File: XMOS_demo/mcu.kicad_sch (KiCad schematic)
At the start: 30 parts, among them J1 XSYS2 DEBUG CONNECTOR, U1 U316-1024-QF60B

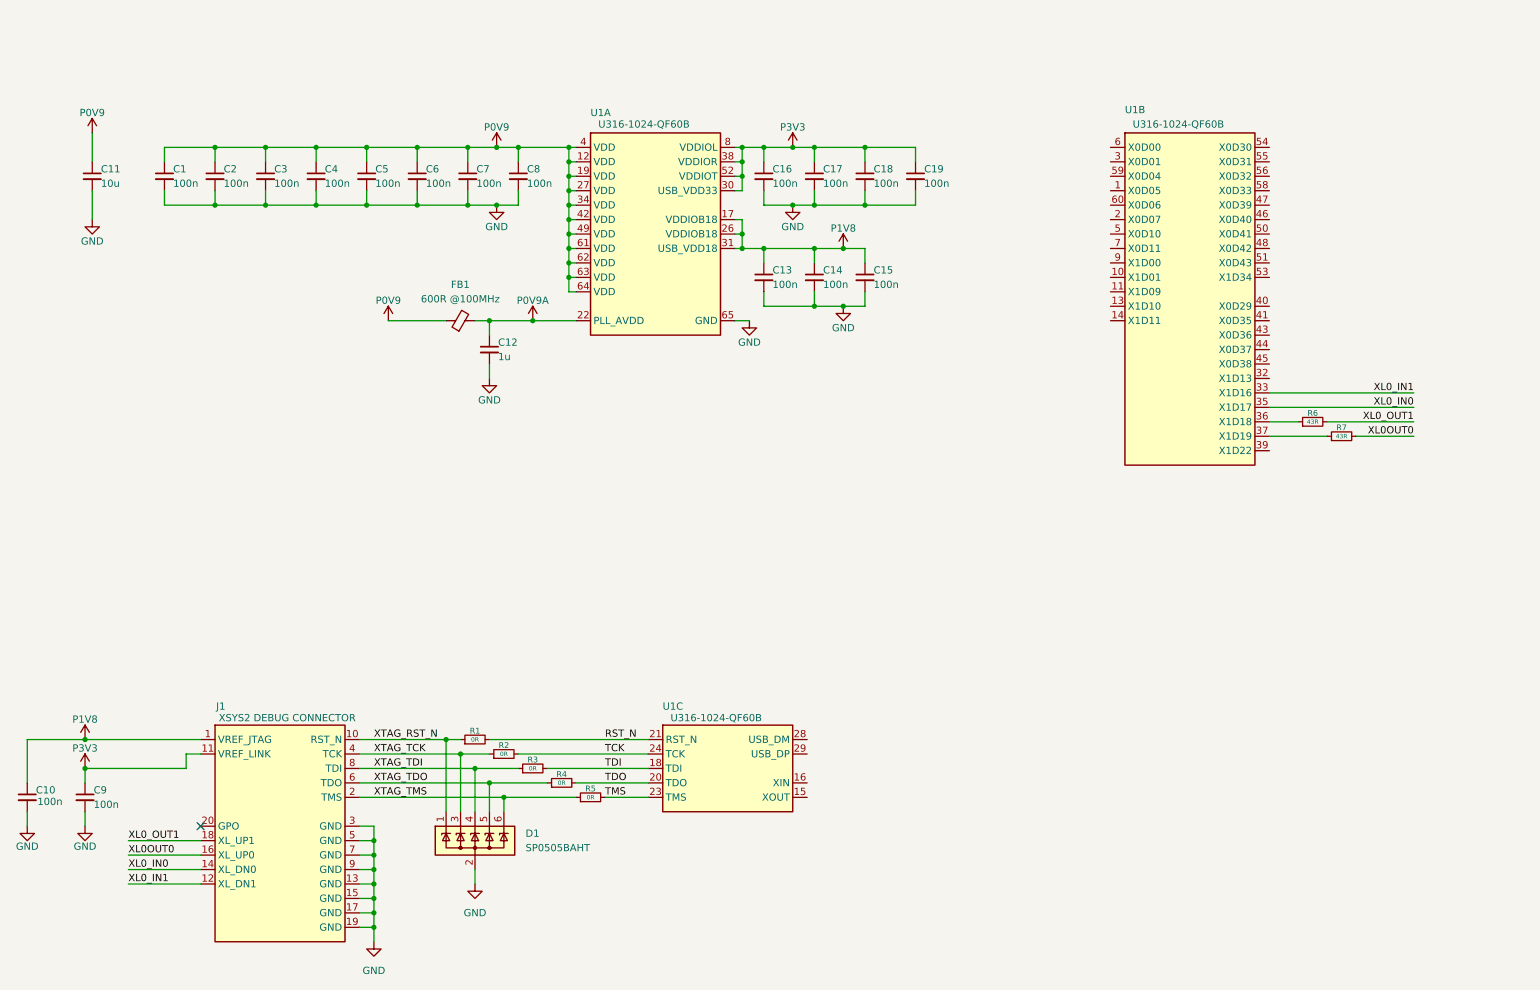
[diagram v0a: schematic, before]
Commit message: crystal, usb
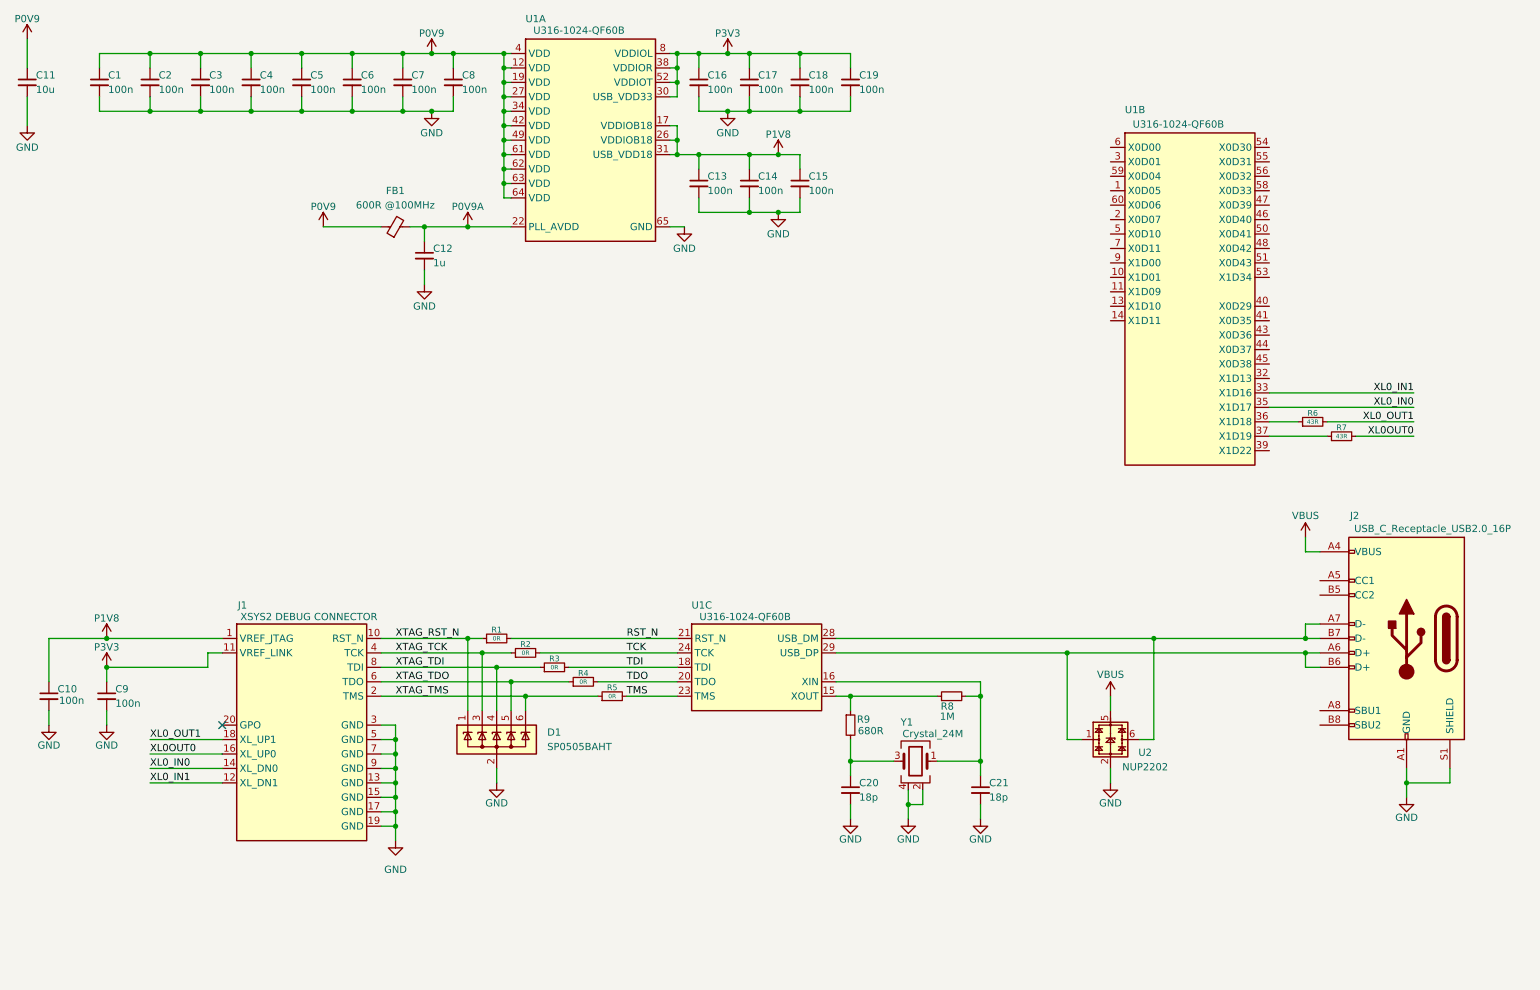
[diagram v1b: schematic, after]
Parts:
- added C20, C21: 18p, Capacitor_SMD:C_0603_1608Metric, symbol Device:C_Small
- added J2: USB_C_Receptacle_USB2.0_16P, Connector_USB:USB_C_Receptacle_GCT_USB4085, symbol Connector:USB_C_Receptacle_USB2.0_16P
- added R8: 1M, Resistor_SMD:R_0603_1608Metric, symbol Device:R_Small
- added R9: 680R, Resistor_SMD:R_0603_1608Metric, symbol Device:R_Small
- added U2: NUP2202, Package_TO_SOT_SMD:SOT-363_SC-70-6, symbol Power_Protection:NUP2202
- added Y1: Crystal_24M, Crystal:Crystal_SMD_2520-4Pin_2.5x2.0mm, symbol _Oscillator:Crystal_24M
- U1: footprint _QFN:QFN-60_7x7mm_P0.4mm_EP_ThermalVias_PowerBars -> _Package_QFN:QFN-60_7x7mm_P0.4mm_EP_ThermalVias_PowerBars
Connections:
- net GND: now also C20.2, C21.2, J2.A1 (GND), J2.A12 (GND), J2.B1 (GND), J2.B12 (GND), J2.S1 (SHIELD), U2.2, Y1.2 (G), Y1.4 (G)
- net at U1.15 (XOUT): now also R8.1, R9.1
- net at U1.16 (XIN): now also C21.1, R8.2, Y1.1
- net at U1.28 (USB_DM): now also J2.A7 (D-), J2.B7 (D-), U2.6
- net at U1.29 (USB_DP): now also J2.A6 (D+), J2.B6 (D+), U2.1
- new net: C20.1, R9.2, Y1.3
- new net VBUS: J2.A4 (VBUS), J2.A9 (VBUS), J2.B4 (VBUS), J2.B9 (VBUS), U2.5
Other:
- moved on the sheet: C1, C10, C11, C12, C13, C14, C15, C16, C17, C18, C19, C2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
